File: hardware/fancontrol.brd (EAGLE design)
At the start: 55 x 50 mm, 11 parts, among them Q1 IRLZ44Z, T1 BC547

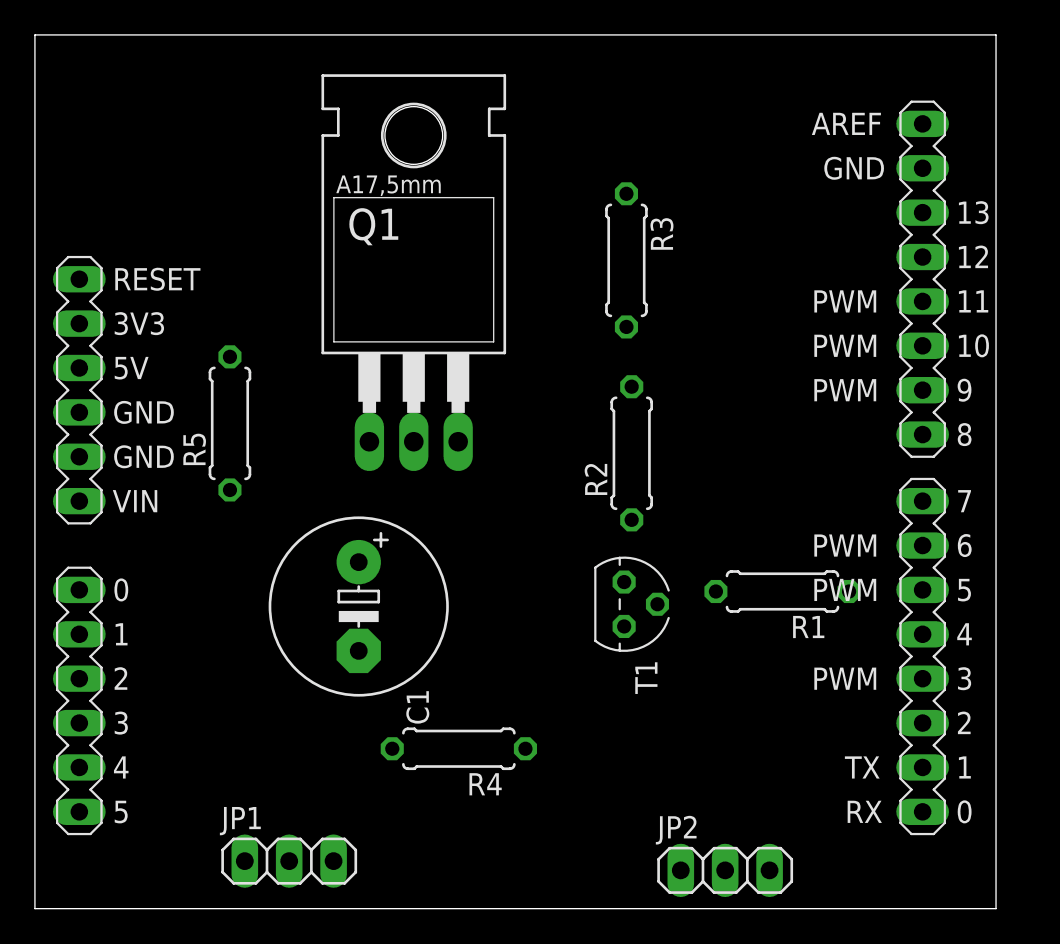
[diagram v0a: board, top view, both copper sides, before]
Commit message: finished the routung
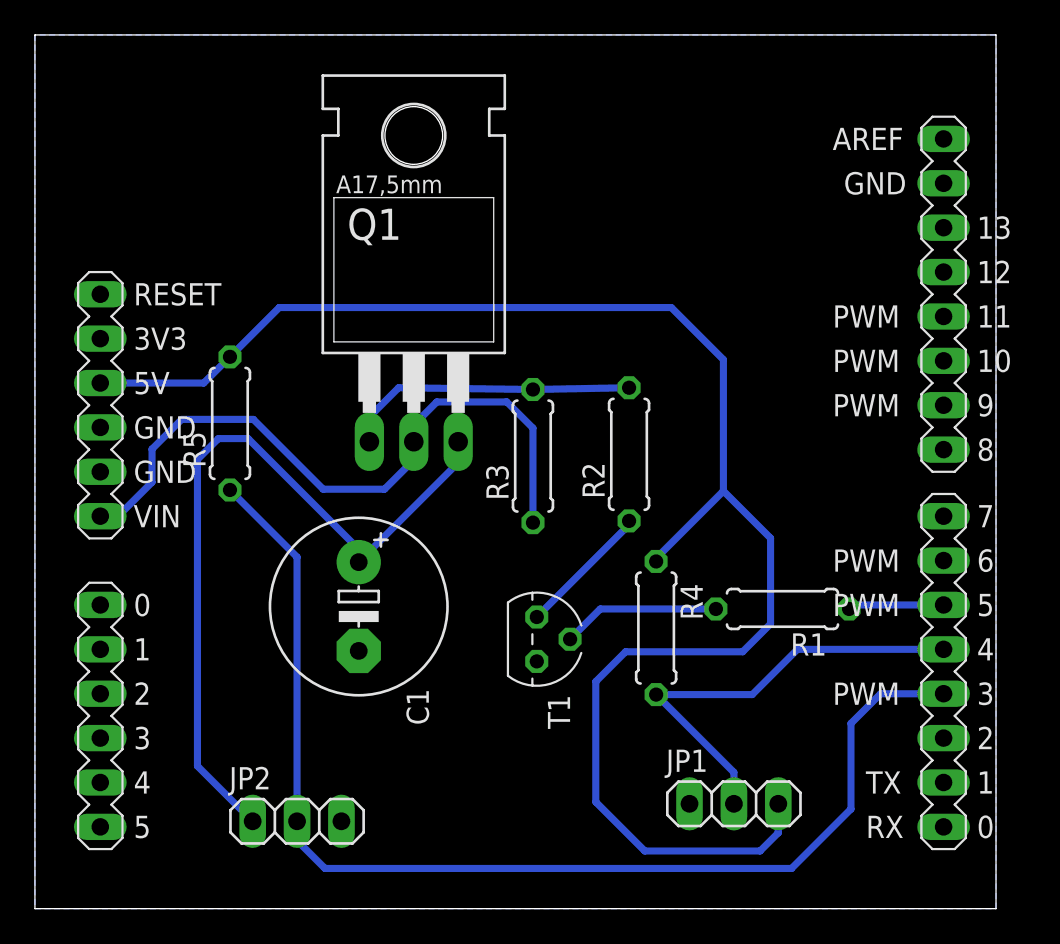
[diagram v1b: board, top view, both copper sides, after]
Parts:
- moved JP1 25.7 mm to (40.0, 6.00)
- moved JP2 24.7 mm to (15.0, 5.00)
- moved R4 13.2 mm to (35.5, 16.1), turned to 270 degrees
- moved R3 12.4 mm to (28.5, 25.9), turned to 90 degrees
- moved T1 5.39 mm to (28.7, 15.4)
- moved ARDUINO1 1.48 mm to (26.6, 25.0)
- moved R1 1.00 mm to (42.8, 17.1)
- moved R2 0.16 mm to (34.0, 26.0)
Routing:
- net +5V: track 0.00 -> 92.5 mm
- net TACHO: track 0.00 -> 66.3 mm
- net FAN+: track 0.00 -> 44.3 mm
- net +12V: track 0.00 -> 39.1 mm
- net DQ: track 0.00 -> 25.6 mm
- net N$3: track 0.00 -> 17.0 mm
- net N$1: track 0.00 -> 9.06 mm
- net N$2: track 0.00 -> 7.69 mm
- net PWM: track 0.00 -> 5.51 mm
- added copper zone on layer 16, net GND
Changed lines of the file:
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@@
 <setting verticaltext="up"/>
 </settings>
-<grid distance="1" unitdist="mm" unit="mm" style="lines" multiple="1" display="no" altdistance="0.025" altunitdist="inch" altunit="inch"/>
+<grid distance="0.1" unitdist="mm" unit="mm" style="lines" multiple="1" display="no" altdistance="0.025" altunitdist="inch" altunit="inch"/>
 <layers>
 <layer number="1" name="Top" color="4" fill="1" visible="yes" active="yes"/>
@@
 <elements>
 <element name="Q1" library="transistor-power" package="TO220BH" value="IRLZ44Z" x="21.68" y="33.07"/>
-<element name="R1" library="rcl" package="0207/7" value="10k" x="42.78" y="18.15" rot="R180"/>
-<element name="T1" library="transistor" package="TO92" value="BC547" x="33.72" y="17.42" rot="R270"/>
-<element name="R2" library="rcl" package="0207/7" value="10k" x="34.15" y="26.06" rot="R90"/>
-<element name="R3" library="rcl" package="0207/7" value="10k" x="33.85" y="37.1" rot="R270"/>
+<element name="R1" library="rcl" package="0207/7" value="10k" x="42.78" y="17.15" rot="R180"/>
+<element name="T1" library="transistor" package="TO92" value="BC547" x="28.72" y="15.42" rot="R270"/>
+<element name="R2" library="rcl" package="0207/7" value="10k" x="34" y="26" rot="R90"/>
+<element name="R3" library="rcl" package="0207/7" value="10k" x="28.5" y="25.9" rot="R90"/>
 <element name="C1" library="rcl" package="E5-10,5" value="470u" x="18.53" y="17.29" rot="R270"/>
-<element name="ARDUINO1" library="arduino" package="ARDUINO" value="ARDUINO" x="25.4" y="25.86"/>
-<element name="JP1" library="pinhead" package="1X03" value="" x="14.55" y="2.72"/>
-<element name="R4" library="rcl" package="0207/7" value="4k7" x="24.26" y="9.15" rot="R180"/>
-<element name="JP2" library="pinhead" package="1X03" value="" x="39.5" y="2.19"/>
+<element name="ARDUINO1" library="arduino" package="ARDUINO" value="ARDUINO" x="26.6" y="25"/>
+<element name="JP1" library="pinhead" package="1X03" value="" x="40" y="6"/>
+<element name="R4" library="rcl" package="0207/7" value="4k7" x="35.55" y="16.06" rot="R270"/>
+<element name="JP2" library="pinhead" package="1X03" value="" x="15" y="5"/>
 <element name="R5" library="rcl" package="0207/7" value="10k" x="11.16" y="27.77" rot="R90"/>
 </elements>
@@
 <contactref element="R1" pad="2"/>
 <contactref element="T1" pad="2"/>
-<wire x1="35.625" y1="17.42" x2="38.97" y2="18.15" width="0" layer="19" extent="1-1"/>
+<wire x1="30.625" y1="15.42" x2="32.355" y2="17.15" width="0.4064" layer="16"/>
+<wire x1="32.355" y1="17.15" x2="38.97" y2="17.15" width="0.4064" layer="16"/>
 </signal>
 <signal name="N$2">
 <contactref element="R2" pad="1"/>
 <contactref element="T1" pad="3"/>
-<wire x1="33.72" y1="18.69" x2="34.15" y2="22.25" width="0" layer="19" extent="1-1"/>
+<wire x1="28.72" y1="16.69" x2="34" y2="21.97" width="0.4064" layer="16"/>
+<wire x1="34" y1="21.97" x2="34" y2="22.19" width="0.4064" layer="16"/>
 </signal>
 <signal name="GND">
@@
 <contactref element="ARDUINO1" pad="GND"/>
 <contactref element="JP1" pad="1"/>
-<wire x1="33.72" y1="16.15" x2="2.54" y2="25.86" width="0" layer="19" extent="1-1"/>
-<wire x1="12.01" y1="2.72" x2="33.72" y2="16.15" width="0" layer="19" extent="1-1"/>
-<wire x1="18.53" y1="14.75" x2="12.01" y2="2.72" width="0" layer="19" extent="1-1"/>
+<polygon width="0.4064" layer="16" isolate="0.4064" orphans="yes">
+<vertex x="0" y="0"/>
+<vertex x="55" y="0"/>
+<vertex x="55" y="50"/>
+<vertex x="0" y="50"/>
+</polygon>
 </signal>
 <signal name="N$3">
@@
 <contactref element="Q1" pad="G"/>
 <contactref element="R3" pad="2"/>
-<wire x1="33.85" y1="33.29" x2="34.15" y2="29.87" width="0" layer="19" extent="1-1"/>
-<wire x1="19.14" y1="26.72" x2="34.15" y2="29.87" width="0" layer="19" extent="1-1"/>
+<wire x1="28.5" y1="29.71" x2="34" y2="29.81" width="0.4064" layer="16"/>
+<wire x1="28.5" y1="29.71" x2="20.81" y2="29.81" width="0.4064" layer="16"/>
+<wire x1="20.81" y1="29.81" x2="19.14" y2="28.14" width="0.4064" layer="16"/>
+<wire x1="19.14" y1="28.14" x2="19.14" y2="26.72" width="0.4064" layer="16"/>
 </signal>
 <signal name="+12V">
@@
 <contactref element="R3" pad="1"/>
 <contactref element="ARDUINO1" pad="VIN"/>
-<wire x1="21.68" y1="26.72" x2="2.54" y2="23.32" width="0" layer="19" extent="1-1"/>
-<wire x1="33.85" y1="40.91" x2="21.68" y2="26.72" width="0" layer="19" extent="1-1"/>
+<wire x1="21.68" y1="26.72" x2="21.68" y2="25.68" width="0.4064" layer="16"/>
+<wire x1="21.68" y1="25.68" x2="20" y2="24" width="0.4064" layer="16"/>
+<wire x1="27" y1="29" x2="23" y2="29" width="0.4064" layer="16"/>
+<wire x1="23" y1="29" x2="21.68" y2="27.68" width="0.4064" layer="16"/>
+<wire x1="21.68" y1="27.68" x2="21.68" y2="26.72" width="0.4064" layer="16"/>
+<wire x1="28.5" y1="22.09" x2="28.5" y2="27.5" width="0.4064" layer="16"/>
+<wire x1="28.5" y1="27.5" x2="27" y2="29" width="0.4064" layer="16"/>
+<wire x1="12.5" y1="28" x2="16.5" y2="24" width="0.4064" layer="16"/>
+<wire x1="16.5" y1="24" x2="20" y2="24" width="0.4064" layer="16"/>
+<wire x1="3.74" y1="22.46" x2="4.76" y2="22.46" width="0.4064" layer="16"/>
+<wire x1="4.76" y1="22.46" x2="6.7" y2="24.4" width="0.4064" layer="16"/>
+<wire x1="6.7" y1="24.4" x2="6.7" y2="26.3" width="0.4064" layer="16"/>
+<wire x1="6.7" y1="26.3" x2="8.4" y2="28" width="0.4064" layer="16"/>
+<wire x1="8.4" y1="28" x2="12.5" y2="28" width="0.4064" layer="16"/>
 </signal>
 <signal name="FAN+">
@@
 <contactref element="C1" pad="+"/>
 <contactref element="JP2" pad="1"/>
-<wire x1="18.53" y1="19.83" x2="36.96" y2="2.19" width="0" layer="19" extent="1-1"/>
-<wire x1="24.22" y1="26.72" x2="18.53" y2="19.83" width="0" layer="19" extent="1-1"/>
+<wire x1="24.22" y1="26.72" x2="24.22" y2="25.52" width="0.4064" layer="16"/>
+<wire x1="24.22" y1="25.52" x2="18.53" y2="19.83" width="0.4064" layer="16"/>
+<wire x1="12.2" y1="26.9" x2="18.53" y2="20.57" width="0.4064" layer="16"/>
+<wire x1="18.53" y1="20.57" x2="18.53" y2="19.83" width="0.4064" layer="16"/>
+<wire x1="12.2" y1="26.9" x2="10.5" y2="26.9" width="0.4064" layer="16"/>
+<wire x1="10.5" y1="26.9" x2="9.3" y2="25.7" width="0.4064" layer="16"/>
+<wire x1="9.3" y1="25.7" x2="9.3" y2="8.16" width="0.4064" layer="16"/>
+<wire x1="9.3" y1="8.16" x2="12.46" y2="5" width="0.4064" layer="16"/>
 </signal>
 <signal name="+5V">
@@
 <contactref element="R4" pad="1"/>
 <contactref element="R5" pad="2"/>
-<wire x1="2.54" y1="30.94" x2="11.16" y2="31.58" width="0" layer="19" extent="1-1"/>
-<wire x1="17.09" y1="2.72" x2="2.54" y2="30.94" width="0" layer="19" extent="1-1"/>
-<wire x1="28.07" y1="9.15" x2="17.09" y2="2.72" width="0" layer="19" extent="1-1"/>
+<wire x1="9.66" y1="30.08" x2="11.16" y2="31.58" width="0.4064" layer="16"/>
+<wire x1="11.16" y1="31.58" x2="13.98" y2="34.4" width="0.4064" layer="16"/>
+<wire x1="13.98" y1="34.4" x2="36.42" y2="34.4" width="0.4064" layer="16"/>
+<wire x1="42.54" y1="6" x2="42.54" y2="4.34" width="0.4064" layer="16"/>
+<wire x1="36.42" y1="34.4" x2="39.4" y2="31.42" width="0.4064" layer="16"/>
+<wire x1="39.4" y1="31.42" x2="39.4" y2="23.9" width="0.4064" layer="16"/>
+<wire x1="39.4" y1="23.9" x2="35.55" y2="20.05" width="0.4064" layer="16"/>
+<wire x1="35.55" y1="20.05" x2="35.55" y2="19.87" width="0.4064" layer="16"/>
+<wire x1="41.5" y1="3.3" x2="34.9" y2="3.3" width="0.4064" layer="16"/>
+<wire x1="40.5" y1="14.7" x2="42.1" y2="16.3" width="0.4064" layer="16"/>
+<wire x1="42.1" y1="16.3" x2="42.1" y2="21.2" width="0.4064" layer="16"/>
+<wire x1="42.1" y1="21.2" x2="39.4" y2="23.9" width="0.4064" layer="16"/>
+<wire x1="41.5" y1="3.3" x2="42.54" y2="4.34" width="0.4064" layer="16"/>
+<wire x1="34.9" y1="3.3" x2="32.1" y2="6.1" width="0.4064" layer="16"/>
+<wire x1="32.1" y1="6.1" x2="32.1" y2="13" width="0.4064" layer="16"/>
+<wire x1="32.1" y1="13" x2="33.8" y2="14.7" width="0.4064" layer="16"/>
+<wire x1="33.8" y1="14.7" x2="40.5" y2="14.7" width="0.4064" layer="16"/>
+<wire x1="3.74" y1="30.08" x2="9.66" y2="30.08" width="0.4064" layer="16"/>
 </signal>
 <signal name="DQ">
@@
 <contactref element="R4" pad="2"/>
 <contactref element="ARDUINO1" pad="04"/>
-<wire x1="14.55" y1="2.72" x2="20.45" y2="9.15" width="0" layer="19" extent="1-1"/>
-<wire x1="50.8" y1="15.7" x2="14.55" y2="2.72" width="0" layer="19" extent="1-1"/>
+<wire x1="40" y1="6" x2="40" y2="7.8" width="0.4064" layer="16"/>
+<wire x1="40" y1="7.8" x2="35.55" y2="12.25" width="0.4064" layer="16"/>
+<wire x1="35.55" y1="12.25" x2="41.05" y2="12.25" width="0.4064" layer="16"/>
+<wire x1="41.05" y1="12.25" x2="43.64" y2="14.84" width="0.4064" layer="16"/>
+<wire x1="43.64" y1="14.84" x2="52" y2="14.84" width="0.4064" layer="16"/>
 </signal>
 <signal name="TACHO">
@@
 <contactref element="JP2" pad="2"/>
 <contactref element="R5" pad="1"/>
-<wire x1="39.5" y1="2.19" x2="11.16" y2="23.96" width="0" layer="19" extent="1-1"/>
-<wire x1="50.8" y1="13.16" x2="39.5" y2="2.19" width="0" layer="19" extent="1-1"/>
+<wire x1="15" y1="5" x2="15" y2="20.12" width="0.4064" layer="16"/>
+<wire x1="15" y1="20.12" x2="11.16" y2="23.96" width="0.4064" layer="16"/>
+<wire x1="48.4" y1="12.3" x2="46.7" y2="10.6" width="0.4064" layer="16"/>
+<wire x1="43.3" y1="2.3" x2="16.6" y2="2.3" width="0.4064" layer="16"/>
+<wire x1="16.6" y1="2.3" x2="15" y2="3.9" width="0.4064" layer="16"/>
+<wire x1="15" y1="3.9" x2="15" y2="5" width="0.4064" layer="16"/>
+<wire x1="43.3" y1="2.3" x2="46.7" y2="5.7" width="0.4064" layer="16"/>
+<wire x1="46.7" y1="5.7" x2="46.7" y2="10.6" width="0.4064" layer="16"/>
+<wire x1="52" y1="12.3" x2="48.4" y2="12.3" width="0.4064" layer="16"/>
 </signal>
 <signal name="PWM">
 <contactref element="ARDUINO1" pad="05"/>
 <contactref element="R1" pad="1"/>
-<wire x1="50.8" y1="18.24" x2="46.59" y2="18.15" width="0" layer="19" extent="1-1"/>
+<wire x1="52" y1="17.38" x2="46.82" y2="17.38" width="0.4064" layer="16"/>
+<wire x1="46.82" y1="17.38" x2="46.59" y2="17.15" width="0.4064" layer="16"/>
 </signal>
 <signal name="N$5">
